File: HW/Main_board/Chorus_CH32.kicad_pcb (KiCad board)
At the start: 2 copper layers, 31.2 x 69.1 mm, 106 parts, among them J1 DC_Jack, J3 SW, J4 IN, J5 OUT, J9 9V, U1 TL072, U2 L78L05_SOT89, U3 TL072, U6 TL072, U8 TL072, U9 CH32V003AxMx

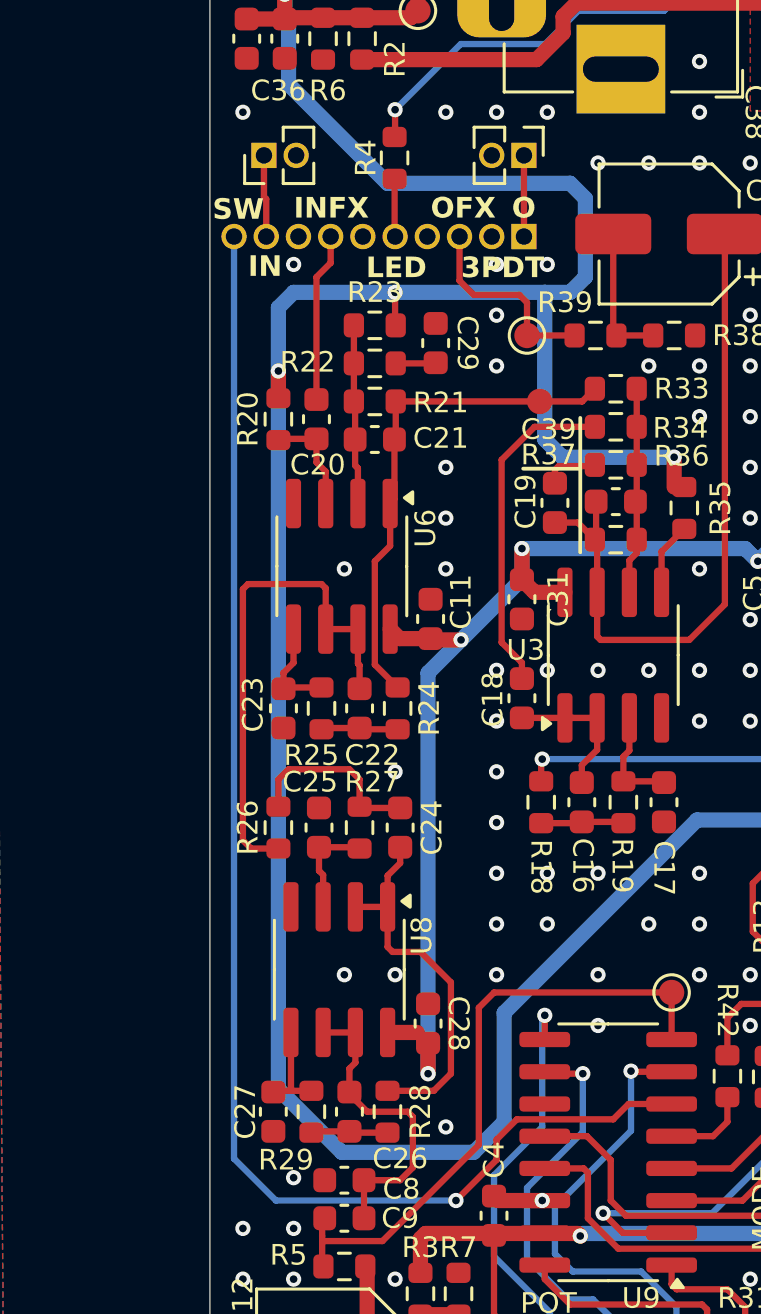
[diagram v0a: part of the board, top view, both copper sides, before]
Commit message: moved spdt connector
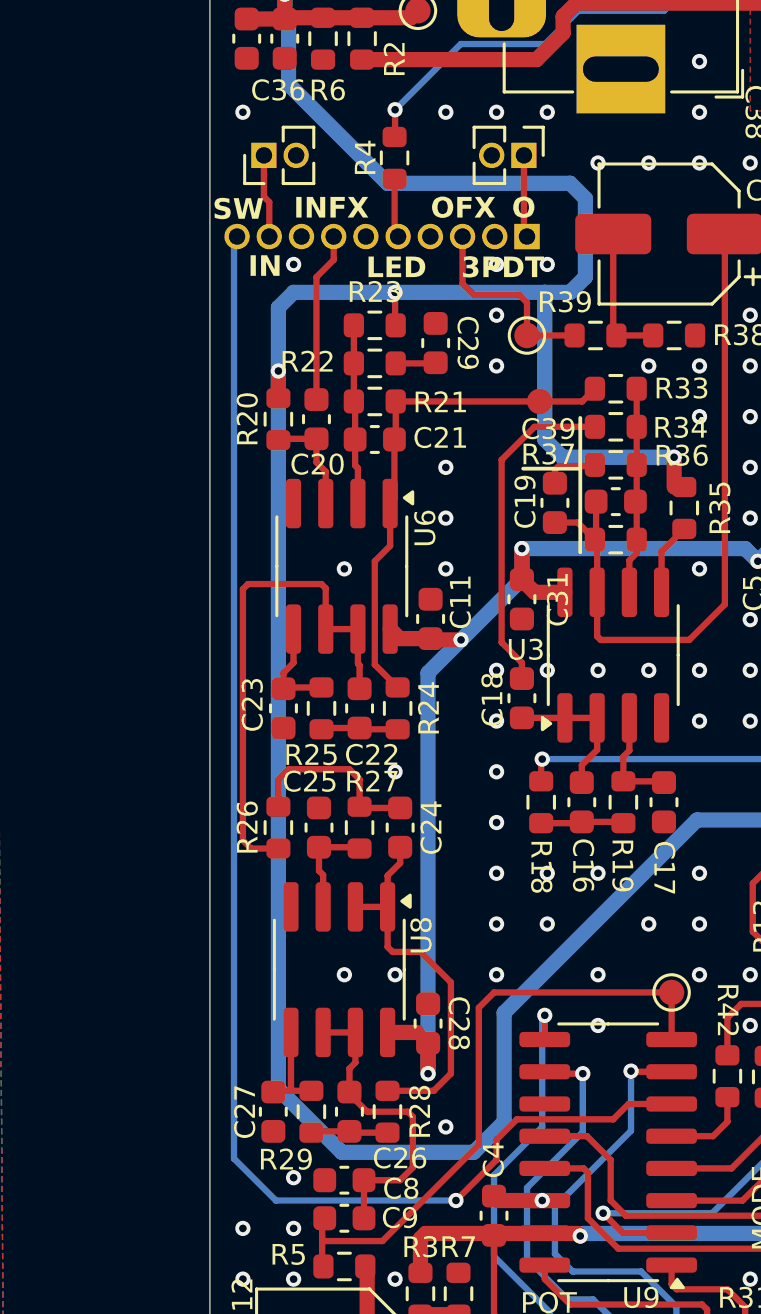
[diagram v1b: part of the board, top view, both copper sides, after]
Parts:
- moved X1 0.12 mm to (145.7, 73.9)
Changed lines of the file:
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@@
 	(footprint "Connector_PinHeader_1.27mm:PinHeader_1x10_P1.27mm_Vertical"
 		(layer "F.Cu")
-		(at 145.58 73.9 -90)
+		(at 145.7 73.9 -90)
 		(descr "Through hole straight pin header, 1x10, 1.27mm pitch, single row")
 		(tags "Through hole pin header THT 1x10 1.27mm single row")
@@
 	)
 	(segment
-		(start 135.42 72.42)
-		(end 135.42 73.9)
+		(start 135.54 72.54)
+		(end 135.54 73.9)
 		(width 0.25)
 		(layer "F.Cu")
@@
 	)
 	(segment
-		(start 135.33 70.7)
-		(end 135.33 72.33)
+		(start 135.33 72.33)
+		(end 135.54 72.54)
 		(width 0.25)
 		(layer "F.Cu")
@@
 	)
 	(segment
-		(start 135.33 72.33)
-		(end 135.42 72.42)
+		(start 135.33 70.7)
+		(end 135.33 72.33)
 		(width 0.25)
 		(layer "F.Cu")
@@
 	)
 	(segment
-		(start 140.48 71.625)
-		(end 140.48 73.88)
+		(start 140.48 73.76)
+		(end 140.62 73.9)
 		(width 0.25)
 		(layer "F.Cu")
@@
 	)
 	(segment
-		(start 140.48 73.88)
-		(end 140.5 73.9)
+		(start 140.48 71.625)
+		(end 140.48 73.76)
 		(width 0.25)
 		(layer "F.Cu")
@@
 	)
 	(segment
-		(start 137.96 73.9)
-		(end 137.96 74.94)
+		(start 138.08 73.9)
+		(end 138.08 74.82)
 		(width 0.25)
 		(layer "F.Cu")
@@
 	)
 	(segment
-		(start 137.96 74.94)
+		(start 138.08 74.82)
 		(end 137.4 75.5)
 		(width 0.25)
@@
 	)
 	(segment
+		(start 145.58 73.78)
+		(end 145.7 73.9)
+		(width 0.25)
+		(layer "F.Cu")
+		(net 13)
+	)
+	(segment
 		(start 145.58 70.7)
-		(end 145.58 73.9)
+		(end 145.58 73.78)
 		(width 0.25)
 		(layer "F.Cu")
@@
 	)
 	(segment
-		(start 135.8 111.9)
-		(end 142.9 111.9)
+		(start 134.15 110.25)
+		(end 135.8 111.9)
 		(width 0.25)
 		(layer "B.Cu")
@@
 	)
 	(segment
-		(start 134.15 110.25)
-		(end 135.8 111.9)
+		(start 134.27 73.9)
+		(end 134.15 74.02)
 		(width 0.25)
 		(layer "B.Cu")
@@
 	)
 	(segment
-		(start 134.15 73.9)
+		(start 134.15 74.02)
 		(end 134.15 110.25)
 		(width 0.25)
@@
 	)
 	(segment
+		(start 135.8 111.9)
+		(end 142.9 111.9)
+		(width 0.25)
+		(layer "B.Cu")
+		(net 34)
+	)
+	(segment
 		(start 153.6 104.7)
 		(end 153.6 106.175)
@@
 	)
 	(segment
-		(start 147.575 77.8)
-		(end 145.7 77.8)
+		(start 145.7 77.8)
+		(end 145.7 76.5)
 		(width 0.25)
 		(layer "F.Cu")
@@
 	)
 	(segment
-		(start 143.04 75.64)
-		(end 143.04 73.9)
+		(start 145.7 76.5)
+		(end 145.4 76.2)
 		(width 0.25)
 		(layer "F.Cu")
@@
 	)
 	(segment
-		(start 145.4 76.2)
-		(end 143.6 76.2)
+		(start 147.575 77.8)
+		(end 145.7 77.8)
 		(width 0.25)
 		(layer "F.Cu")
@@
 	(segment
 		(start 143.6 76.2)
-		(end 143.04 75.64)
+		(end 143.16 75.76)
 		(width 0.25)
 		(layer "F.Cu")
@@
 	)
 	(segment
-		(start 145.7 76.5)
-		(end 145.4 76.2)
+		(start 145.4 76.2)
+		(end 143.6 76.2)
 		(width 0.25)
 		(layer "F.Cu")
@@
 	)
 	(segment
-		(start 145.7 77.8)
-		(end 145.7 76.5)
+		(start 143.16 75.76)
+		(end 143.16 73.9)
 		(width 0.25)
 		(layer "F.Cu")
